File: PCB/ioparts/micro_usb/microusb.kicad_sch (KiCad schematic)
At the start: 2 parts, among them J1 USB_B_Micro, J3 Conn_01x04

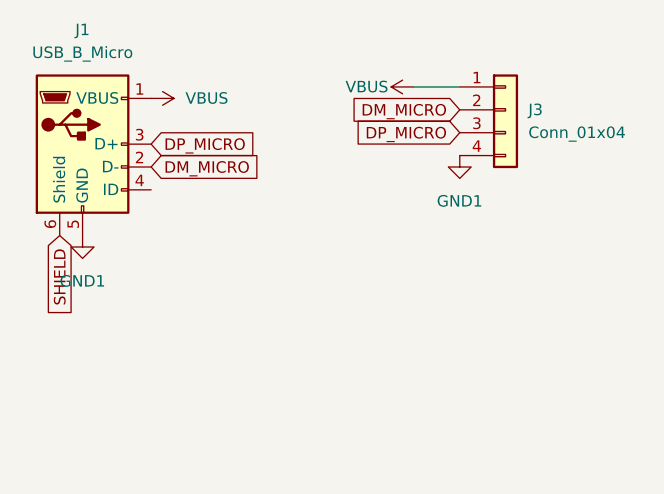
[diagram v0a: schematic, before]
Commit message: misc pcbs
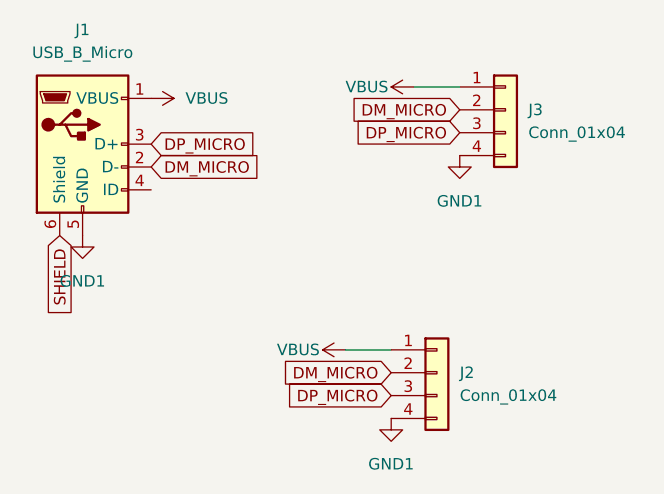
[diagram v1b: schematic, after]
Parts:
- added J2: Conn_01x04, Connector_JST:JST_SH_SM04B-SRSS-TB_1x04-1MP_P1.00mm_Horizontal, symbol Connector_Generic:Conn_01x04
- J1: footprint Connector_USB:USB_Micro-B_Amphenol_10118194_Horizontal -> ioparts:HRO_U-G-M5WS-W-01
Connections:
- net DM_MICRO: now also J2.2 (Pin_2)
- net DP_MICRO: now also J2.3 (Pin_3)
- net GND1: now also J2.4 (Pin_4)
- net VBUS: now also J2.1 (Pin_1)
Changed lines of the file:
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@@
 (kicad_sch (version 20211123) (generator eeschema)
   (paper "A4")
+  (wire (pts (xy 100.33 138.43) (xy 105.41 138.43))
+    (stroke (width 0) (type default) (color 0 0 0 0))
+  )
   (wire (pts (xy 107.95 109.22) (xy 113.03 109.22))
     (stroke (width 0) (type default) (color 0 0 0 0))
@@
     )
   )
+  (global_label "DM_MICRO" (shape input) (at 105.41 140.97 180) (fields_autoplaced)
+    (effects (font (size 1.27 1.27)) (justify right))
+    (property "Intersheet References" "${INTERSHEET_REFS}" (id 0) (at 93.3812 140.8906 0)
+      (effects (font (size 1.27 1.27)) (justify right) hide)
+    )
+  )
   (global_label "DM_MICRO" (shape input) (at 113.03 111.76 180) (fields_autoplaced)
     (effects (font (size 1.27 1.27)) (justify right))
     (property "Intersheet References" "${INTERSHEET_REFS}" (id 0) (at 101.0012 111.6806 0)
+      (effects (font (size 1.27 1.27)) (justify right) hide)
+    )
+  )
+  (global_label "DP_MICRO" (shape input) (at 105.41 143.51 180) (fields_autoplaced)
+    (effects (font (size 1.27 1.27)) (justify right))
+    (property "Intersheet References" "${INTERSHEET_REFS}" (id 0) (at 93.5626 143.4306 0)
       (effects (font (size 1.27 1.27)) (justify right) hide)
     )
@@
     )
   )
+  (symbol (lib_id "power:VBUS") (at 100.33 138.43 90) (unit 1)
+    (in_bom yes) (on_board yes)
+    (property "Reference" "#PWR0105" (id 0) (at 104.14 138.43 0)
+      (effects (font (size 1.27 1.27)) hide)
+    )
+    (property "Value" "VBUS" (id 1) (at 92.71 138.43 90)
+      (effects (font (size 1.27 1.27)) (justify right))
+    )
+    (property "Footprint" "" (id 2) (at 100.33 138.43 0)
+      (effects (font (size 1.27 1.27)) hide)
+    )
+    (property "Datasheet" "" (id 3) (at 100.33 138.43 0)
+      (effects (font (size 1.27 1.27)) hide)
+    )
+    (pin "1")
+  )
   (symbol (lib_id "power:GND1") (at 113.03 116.84 0) (unit 1)
     (in_bom yes) (on_board yes) (fields_autoplaced)
@@
   (symbol (lib_id "power:VBUS") (at 107.95 109.22 90) (unit 1)
     (in_bom yes) (on_board yes)
-    (property "Reference" "#PWR?" (id 0) (at 111.76 109.22 0)
+    (property "Reference" "#PWR0102" (id 0) (at 111.76 109.22 0)
       (effects (font (size 1.27 1.27)) hide)
     )
@@
     (pin "1")
   )
+  (symbol (lib_id "Connector_Generic:Conn_01x04") (at 110.49 140.97 0) (unit 1)
+    (in_bom yes) (on_board yes) (fields_autoplaced)
+    (property "Reference" "J2" (id 0) (at 113.03 140.9699 0)
+      (effects (font (size 1.27 1.27)) (justify left))
+    )
+    (property "Value" "Conn_01x04" (id 1) (at 113.03 143.5099 0)
+      (effects (font (size 1.27 1.27)) (justify left))
+    )
+    (property "Footprint" "Connector_JST:JST_SH_SM04B-SRSS-TB_1x04-1MP_P1.00mm_Horizontal" (id 2) (at 110.49 140.97 0)
+      (effects (font (size 1.27 1.27)) hide)
+    )
+    (property "Datasheet" "~" (id 3) (at 110.49 140.97 0)
+      (effects (font (size 1.27 1.27)) hide)
+    )
+    (pin "1")
+    (pin "2")
+    (pin "3")
+    (pin "4")
+  )
   (symbol (lib_id "power:VBUS") (at 78.74 110.49 270) (unit 1)
     (in_bom yes) (on_board yes) (fields_autoplaced)
@@
     (property "Reference" "J1" (id 0) (at 71.12 102.87 0))
     (property "Value" "USB_B_Micro" (id 1) (at 71.12 105.41 0))
-    (property "Footprint" "Connector_USB:USB_Micro-B_Amphenol_10118194_Horizontal" (id 2) (at 74.93 116.84 0)
+    (property "Footprint" "ioparts:HRO_U-G-M5WS-W-01" (id 2) (at 74.93 116.84 0)
       (effects (font (size 1.27 1.27)) hide)
     )
@@
     (pin "4")
   )
+  (symbol (lib_id "power:GND1") (at 105.41 146.05 0) (unit 1)
+    (in_bom yes) (on_board yes) (fields_autoplaced)
+    (property "Reference" "#PWR0104" (id 0) (at 105.41 152.4 0)
+      (effects (font (size 1.27 1.27)) hide)
+    )
+    (property "Value" "GND1" (id 1) (at 105.41 151.13 0))
+    (property "Footprint" "" (id 2) (at 105.41 146.05 0)
+      (effects (font (size 1.27 1.27)) hide)
+    )
+    (property "Datasheet" "" (id 3) (at 105.41 146.05 0)
+      (effects (font (size 1.27 1.27)) hide)
+    )
+    (pin "1")
+  )
   (sheet_instances
     (path "/" (page "1"))
@@
       (reference "#PWR0101") (unit 1) (value "GND1") (footprint "")
     )
+    (path "/3419c53e-5d72-4908-96e4-826d8e519ee8"
+      (reference "#PWR0102") (unit 1) (value "VBUS") (footprint "")
+    )
     (path "/4ede8836-129e-4219-b1ac-6ee8f77f8f88"
       (reference "#PWR0103") (unit 1) (value "VBUS") (footprint "")
     )
+    (path "/f9f24c65-6c35-4cf6-8dc1-d79017c03d44"
+      (reference "#PWR0104") (unit 1) (value "GND1") (footprint "")
+    )
+    (path "/08c035b9-99c4-41cd-8f47-56dfb2fdee80"
+      (reference "#PWR0105") (unit 1) (value "VBUS") (footprint "")
+    )
     (path "/24c540f6-4419-4fc4-bc4f-902d0a711339"
       (reference "#PWR0106") (unit 1) (value "GND1") (footprint "")
     )
-    (path "/3419c53e-5d72-4908-96e4-826d8e519ee8"
-      (reference "#PWR?") (unit 1) (value "VBUS") (footprint "")
-    )
     (path "/78e39353-88dc-4233-86f2-5db925308c49"
-      (reference "J1") (unit 1) (value "USB_B_Micro") (footprint "Connector_USB:USB_Micro-B_Amphenol_10118194_Horizontal")
+      (reference "J1") (unit 1) (value "USB_B_Micro") (footprint "ioparts:HRO_U-G-M5WS-W-01")
+    )
+    (path "/46e403d7-c7fe-4047-b9c1-8a4bf2fc57cd"
+      (reference "J2") (unit 1) (value "Conn_01x04") (footprint "Connector_JST:JST_SH_SM04B-SRSS-TB_1x04-1MP_P1.00mm_Horizontal")
     )
     (path "/b9a92b39-e387-41bf-9641-9883e116b75e"
